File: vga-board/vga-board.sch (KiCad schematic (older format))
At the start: 44 parts, among them J1 Conn_02x20_Odd_Even, J2 Conn_02x20_Odd_Even, J3 DB15_Female_HighDensity, U1 74HC244, U10 74HC163, U11 74LS158, U12 74LS251, U13 74HC244, U14 74HC244, U15 74HC244, U16 GAL22V10, U17 GAL22V10, U18 GAL22V10, U19 74HC163, U2 74HC373, U20 74HC163, U21 74HC163, U22 74HC163, U23 74HC163, U3 74HC244, U4 74HC373, U5 74HC373, U6 74HC373, U7 74HC373, U8 71256SA12TPG, U9 74HC244, X1 40MHz

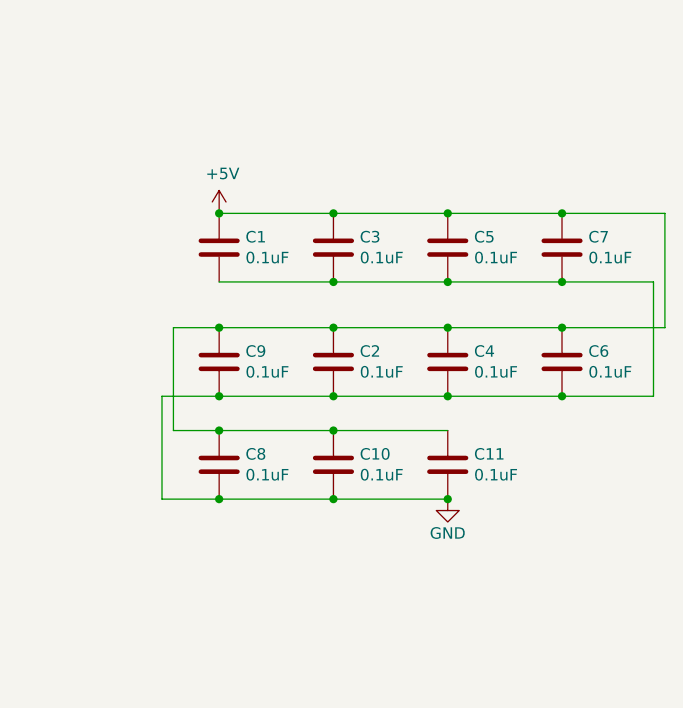
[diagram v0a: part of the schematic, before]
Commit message: Revert "More on layouts"
This reverts commit 3fc7c4d1a32f245eaa0a26aebed00be081417dbd.
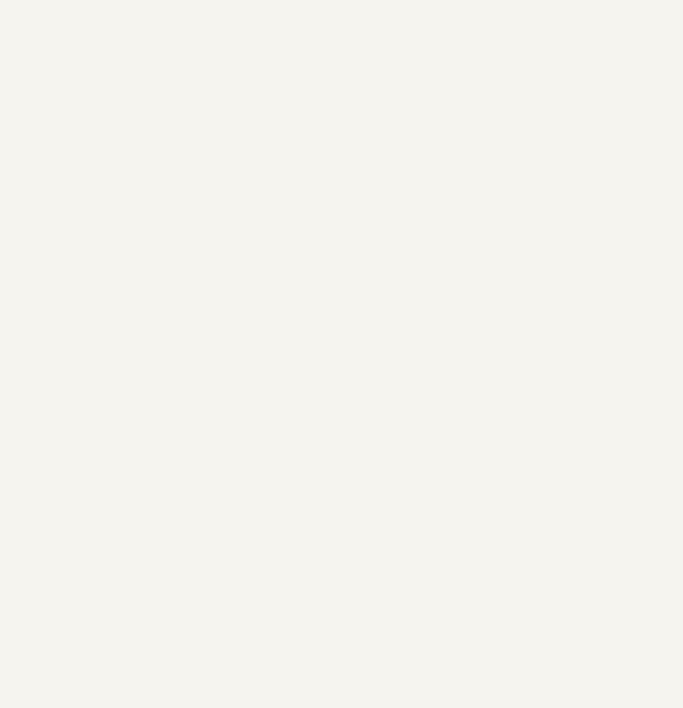
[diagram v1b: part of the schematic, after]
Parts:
- removed C1, C10, C11, C2, C3, C4, C5, C6, C7, C8, C9: 0.1uF, Capacitor_THT:C_Disc_D6.0mm_W2.5mm_P5.00mm, symbol Device:C
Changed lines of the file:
@@
 $EndComp
 NoConn ~ 14850 8500
-$Comp
-L Device:C C1
-U 1 1 5FE43840
-P 16900 2350
-F 0 "C1" H 17015 2396 50  0000 L CNN
-F 1 "0.1uF" H 17015 2305 50  0000 L CNN
-F 2 "Capacitor_THT:C_Disc_D6.0mm_W2.5mm_P5.00mm" H 16938 2200 50  0001 C CNN
-F 3 "~" H 16900 2350 50  0001 C CNN
-	1    16900 2350
-	1    0    0    -1
-$EndComp
-$Comp
-L Device:C C3
-U 1 1 5FE455E8
-P 17400 2350
-F 0 "C3" H 17515 2396 50  0000 L CNN
-F 1 "0.1uF" H 17515 2305 50  0000 L CNN
-F 2 "Capacitor_THT:C_Disc_D6.0mm_W2.5mm_P5.00mm" H 17438 2200 50  0001 C CNN
-F 3 "~" H 17400 2350 50  0001 C CNN
-	1    17400 2350
-	1    0    0    -1
-$EndComp
-$Comp
-L Device:C C5
-U 1 1 5FE4566B
-P 17900 2350
-F 0 "C5" H 18015 2396 50  0000 L CNN
-F 1 "0.1uF" H 18015 2305 50  0000 L CNN
-F 2 "Capacitor_THT:C_Disc_D6.0mm_W2.5mm_P5.00mm" H 17938 2200 50  0001 C CNN
-F 3 "~" H 17900 2350 50  0001 C CNN
-	1    17900 2350
-	1    0    0    -1
-$EndComp
-$Comp
-L Device:C C7
-U 1 1 5FE456D2
-P 18400 2350
-F 0 "C7" H 18515 2396 50  0000 L CNN
-F 1 "0.1uF" H 18515 2305 50  0000 L CNN
-F 2 "Capacitor_THT:C_Disc_D6.0mm_W2.5mm_P5.00mm" H 18438 2200 50  0001 C CNN
-F 3 "~" H 18400 2350 50  0001 C CNN
-	1    18400 2350
-	1    0    0    -1
-$EndComp
-$Comp
-L Device:C C9
-U 1 1 5FE45727
-P 16900 2850
-F 0 "C9" H 17015 2896 50  0000 L CNN
-F 1 "0.1uF" H 17015 2805 50  0000 L CNN
-F 2 "Capacitor_THT:C_Disc_D6.0mm_W2.5mm_P5.00mm" H 16938 2700 50  0001 C CNN
-F 3 "~" H 16900 2850 50  0001 C CNN
-	1    16900 2850
-	1    0    0    -1
-$EndComp
-$Comp
-L Device:C C2
-U 1 1 5FE4577C
-P 17400 2850
-F 0 "C2" H 17515 2896 50  0000 L CNN
-F 1 "0.1uF" H 17515 2805 50  0000 L CNN
-F 2 "Capacitor_THT:C_Disc_D6.0mm_W2.5mm_P5.00mm" H 17438 2700 50  0001 C CNN
-F 3 "~" H 17400 2850 50  0001 C CNN
-	1    17400 2850
-	1    0    0    -1
-$EndComp
-$Comp
-L Device:C C4
-U 1 1 5FE457D6
-P 17900 2850
-F 0 "C4" H 18015 2896 50  0000 L CNN
-F 1 "0.1uF" H 18015 2805 50  0000 L CNN
-F 2 "Capacitor_THT:C_Disc_D6.0mm_W2.5mm_P5.00mm" H 17938 2700 50  0001 C CNN
-F 3 "~" H 17900 2850 50  0001 C CNN
-	1    17900 2850
-	1    0    0    -1
-$EndComp
-$Comp
-L Device:C C6
-U 1 1 5FE45854
-P 18400 2850
-F 0 "C6" H 18515 2896 50  0000 L CNN
-F 1 "0.1uF" H 18515 2805 50  0000 L CNN
-F 2 "Capacitor_THT:C_Disc_D6.0mm_W2.5mm_P5.00mm" H 18438 2700 50  0001 C CNN
-F 3 "~" H 18400 2850 50  0001 C CNN
-	1    18400 2850
-	1    0    0    -1
-$EndComp
-$Comp
-L Device:C C8
-U 1 1 5FE458A9
-P 16900 3300
-F 0 "C8" H 17015 3346 50  0000 L CNN
-F 1 "0.1uF" H 17015 3255 50  0000 L CNN
-F 2 "Capacitor_THT:C_Disc_D6.0mm_W2.5mm_P5.00mm" H 16938 3150 50  0001 C CNN
-F 3 "~" H 16900 3300 50  0001 C CNN
-	1    16900 3300
-	1    0    0    -1
-$EndComp
-$Comp
-L Device:C C10
-U 1 1 5FE458FE
-P 17400 3300
-F 0 "C10" H 17515 3346 50  0000 L CNN
-F 1 "0.1uF" H 17515 3255 50  0000 L CNN
-F 2 "Capacitor_THT:C_Disc_D6.0mm_W2.5mm_P5.00mm" H 17438 3150 50  0001 C CNN
-F 3 "~" H 17400 3300 50  0001 C CNN
-	1    17400 3300
-	1    0    0    -1
-$EndComp
-$Comp
-L Device:C C11
-U 1 1 5FE9F61C
-P 17900 3300
-F 0 "C11" H 18015 3346 50  0000 L CNN
-F 1 "0.1uF" H 18015 3255 50  0000 L CNN
-F 2 "Capacitor_THT:C_Disc_D6.0mm_W2.5mm_P5.00mm" H 17938 3150 50  0001 C CNN
-F 3 "~" H 17900 3300 50  0001 C CNN
-	1    17900 3300
-	1    0    0    -1
-$EndComp
-Wire Wire Line
-	16900 2200 17400 2200
-Connection ~ 17400 2200
-Wire Wire Line
-	17400 2200 17900 2200
-Connection ~ 17900 2200
-Wire Wire Line
-	17900 2200 18400 2200
-Wire Wire Line
-	18400 2200 18850 2200
-Wire Wire Line
-	18850 2200 18850 2700
-Wire Wire Line
-	18850 2700 18400 2700
-Connection ~ 18400 2200
-Connection ~ 17900 2700
-Wire Wire Line
-	17900 2700 17400 2700
-Connection ~ 18400 2700
-Wire Wire Line
-	18400 2700 17900 2700
-Wire Wire Line
-	17400 2700 16900 2700
-Wire Wire Line
-	16700 2700 16700 3150
-Wire Wire Line
-	16700 3150 16900 3150
-Connection ~ 17400 2700
-Connection ~ 16900 2700
-Wire Wire Line
-	16900 2700 16700 2700
-Connection ~ 16900 3150
-Wire Wire Line
-	16900 3150 17400 3150
-Connection ~ 17400 3150
-Wire Wire Line
-	17400 3150 17900 3150
-Wire Wire Line
-	16900 2500 17400 2500
-Wire Wire Line
-	18800 2500 18800 3000
-Wire Wire Line
-	18800 3000 18400 3000
-Wire Wire Line
-	16650 3000 16650 3450
-Wire Wire Line
-	16650 3450 16900 3450
-Connection ~ 17400 2500
-Wire Wire Line
-	17400 2500 17900 2500
-Connection ~ 17900 2500
-Wire Wire Line
-	17900 2500 18400 2500
-Connection ~ 18400 2500
-Wire Wire Line
-	18400 2500 18800 2500
-Connection ~ 16900 3000
-Wire Wire Line
-	16900 3000 16650 3000
-Connection ~ 17400 3000
-Wire Wire Line
-	17400 3000 16900 3000
-Connection ~ 17900 3000
-Wire Wire Line
-	17900 3000 17400 3000
-Connection ~ 18400 3000
-Wire Wire Line
-	18400 3000 17900 3000
-Connection ~ 16900 3450
-Wire Wire Line
-	16900 3450 17400 3450
-Connection ~ 17400 3450
-Wire Wire Line
-	17400 3450 17900 3450
-Connection ~ 17900 3450
-$Comp
-L power:+5V #PWR0173
-U 1 1 5FEBEE51
-P 16900 2200
-F 0 "#PWR0173" H 16900 2050 50  0001 C CNN
-F 1 "+5V" H 16915 2373 50  0000 C CNN
-F 2 "" H 16900 2200 50  0001 C CNN
-F 3 "" H 16900 2200 50  0001 C CNN
-	1    16900 2200
-	1    0    0    -1
-$EndComp
-Connection ~ 16900 2200
-$Comp
-L power:GND #PWR0174
-U 1 1 5FEBF844
-P 17900 3450
-F 0 "#PWR0174" H 17900 3200 50  0001 C CNN
-F 1 "GND" H 17900 3300 50  0000 C CNN
-F 2 "" H 17900 3450 50  0001 C CNN
-F 3 "" H 17900 3450 50  0001 C CNN
-	1    17900 3450
-	1    0    0    -1
-$EndComp
 $EndSCHEMATC

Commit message: More on layouts
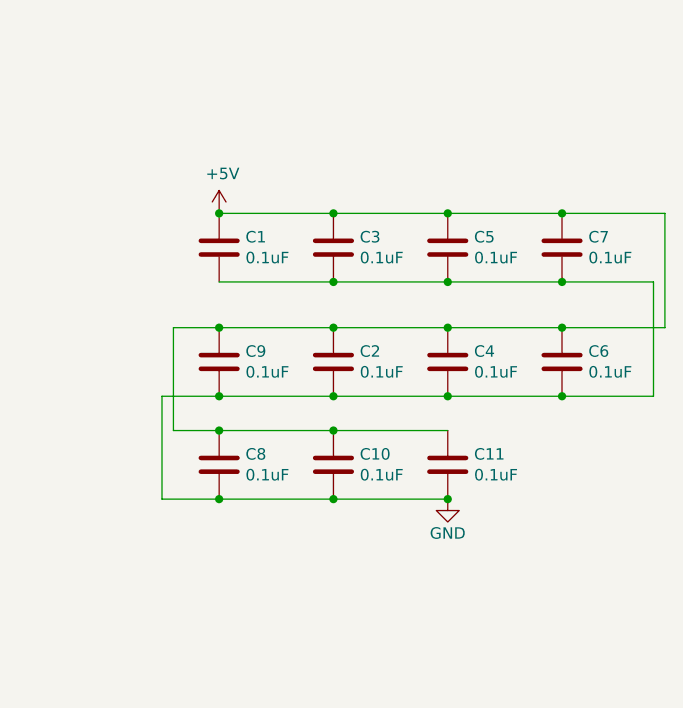
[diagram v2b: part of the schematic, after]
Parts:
- added C1, C10, C11, C2, C3, C4, C5, C6, C7, C8, C9: 0.1uF, Capacitor_THT:C_Disc_D6.0mm_W2.5mm_P5.00mm, symbol Device:C
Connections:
- net +5V: now also C1.1, C10.1, C11.1, C2.1, C3.1, C4.1, C5.1, C6.1, C7.1, C8.1, C9.1
- net GND: now also C1.2, C10.2, C11.2, C2.2, C3.2, C4.2, C5.2, C6.2, C7.2, C8.2, C9.2
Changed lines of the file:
@@
 $EndComp
 NoConn ~ 14850 8500
+$Comp
+L Device:C C1
+U 1 1 5FE43840
+P 16900 2350
+F 0 "C1" H 17015 2396 50  0000 L CNN
+F 1 "0.1uF" H 17015 2305 50  0000 L CNN
+F 2 "Capacitor_THT:C_Disc_D6.0mm_W2.5mm_P5.00mm" H 16938 2200 50  0001 C CNN
+F 3 "~" H 16900 2350 50  0001 C CNN
+	1    16900 2350
+	1    0    0    -1
+$EndComp
+$Comp
+L Device:C C3
+U 1 1 5FE455E8
+P 17400 2350
+F 0 "C3" H 17515 2396 50  0000 L CNN
+F 1 "0.1uF" H 17515 2305 50  0000 L CNN
+F 2 "Capacitor_THT:C_Disc_D6.0mm_W2.5mm_P5.00mm" H 17438 2200 50  0001 C CNN
+F 3 "~" H 17400 2350 50  0001 C CNN
+	1    17400 2350
+	1    0    0    -1
+$EndComp
+$Comp
+L Device:C C5
+U 1 1 5FE4566B
+P 17900 2350
+F 0 "C5" H 18015 2396 50  0000 L CNN
+F 1 "0.1uF" H 18015 2305 50  0000 L CNN
+F 2 "Capacitor_THT:C_Disc_D6.0mm_W2.5mm_P5.00mm" H 17938 2200 50  0001 C CNN
+F 3 "~" H 17900 2350 50  0001 C CNN
+	1    17900 2350
+	1    0    0    -1
+$EndComp
+$Comp
+L Device:C C7
+U 1 1 5FE456D2
+P 18400 2350
+F 0 "C7" H 18515 2396 50  0000 L CNN
+F 1 "0.1uF" H 18515 2305 50  0000 L CNN
+F 2 "Capacitor_THT:C_Disc_D6.0mm_W2.5mm_P5.00mm" H 18438 2200 50  0001 C CNN
+F 3 "~" H 18400 2350 50  0001 C CNN
+	1    18400 2350
+	1    0    0    -1
+$EndComp
+$Comp
+L Device:C C9
+U 1 1 5FE45727
+P 16900 2850
+F 0 "C9" H 17015 2896 50  0000 L CNN
+F 1 "0.1uF" H 17015 2805 50  0000 L CNN
+F 2 "Capacitor_THT:C_Disc_D6.0mm_W2.5mm_P5.00mm" H 16938 2700 50  0001 C CNN
+F 3 "~" H 16900 2850 50  0001 C CNN
+	1    16900 2850
+	1    0    0    -1
+$EndComp
+$Comp
+L Device:C C2
+U 1 1 5FE4577C
+P 17400 2850
+F 0 "C2" H 17515 2896 50  0000 L CNN
+F 1 "0.1uF" H 17515 2805 50  0000 L CNN
+F 2 "Capacitor_THT:C_Disc_D6.0mm_W2.5mm_P5.00mm" H 17438 2700 50  0001 C CNN
+F 3 "~" H 17400 2850 50  0001 C CNN
+	1    17400 2850
+	1    0    0    -1
+$EndComp
+$Comp
+L Device:C C4
+U 1 1 5FE457D6
+P 17900 2850
+F 0 "C4" H 18015 2896 50  0000 L CNN
+F 1 "0.1uF" H 18015 2805 50  0000 L CNN
+F 2 "Capacitor_THT:C_Disc_D6.0mm_W2.5mm_P5.00mm" H 17938 2700 50  0001 C CNN
+F 3 "~" H 17900 2850 50  0001 C CNN
+	1    17900 2850
+	1    0    0    -1
+$EndComp
+$Comp
+L Device:C C6
+U 1 1 5FE45854
+P 18400 2850
+F 0 "C6" H 18515 2896 50  0000 L CNN
+F 1 "0.1uF" H 18515 2805 50  0000 L CNN
+F 2 "Capacitor_THT:C_Disc_D6.0mm_W2.5mm_P5.00mm" H 18438 2700 50  0001 C CNN
+F 3 "~" H 18400 2850 50  0001 C CNN
+	1    18400 2850
+	1    0    0    -1
+$EndComp
+$Comp
+L Device:C C8
+U 1 1 5FE458A9
+P 16900 3300
+F 0 "C8" H 17015 3346 50  0000 L CNN
+F 1 "0.1uF" H 17015 3255 50  0000 L CNN
+F 2 "Capacitor_THT:C_Disc_D6.0mm_W2.5mm_P5.00mm" H 16938 3150 50  0001 C CNN
+F 3 "~" H 16900 3300 50  0001 C CNN
+	1    16900 3300
+	1    0    0    -1
+$EndComp
+$Comp
+L Device:C C10
+U 1 1 5FE458FE
+P 17400 3300
+F 0 "C10" H 17515 3346 50  0000 L CNN
+F 1 "0.1uF" H 17515 3255 50  0000 L CNN
+F 2 "Capacitor_THT:C_Disc_D6.0mm_W2.5mm_P5.00mm" H 17438 3150 50  0001 C CNN
+F 3 "~" H 17400 3300 50  0001 C CNN
+	1    17400 3300
+	1    0    0    -1
+$EndComp
+$Comp
+L Device:C C11
+U 1 1 5FE9F61C
+P 17900 3300
+F 0 "C11" H 18015 3346 50  0000 L CNN
+F 1 "0.1uF" H 18015 3255 50  0000 L CNN
+F 2 "Capacitor_THT:C_Disc_D6.0mm_W2.5mm_P5.00mm" H 17938 3150 50  0001 C CNN
+F 3 "~" H 17900 3300 50  0001 C CNN
+	1    17900 3300
+	1    0    0    -1
+$EndComp
+Wire Wire Line
+	16900 2200 17400 2200
+Connection ~ 17400 2200
+Wire Wire Line
+	17400 2200 17900 2200
+Connection ~ 17900 2200
+Wire Wire Line
+	17900 2200 18400 2200
+Wire Wire Line
+	18400 2200 18850 2200
+Wire Wire Line
+	18850 2200 18850 2700
+Wire Wire Line
+	18850 2700 18400 2700
+Connection ~ 18400 2200
+Connection ~ 17900 2700
+Wire Wire Line
+	17900 2700 17400 2700
+Connection ~ 18400 2700
+Wire Wire Line
+	18400 2700 17900 2700
+Wire Wire Line
+	17400 2700 16900 2700
+Wire Wire Line
+	16700 2700 16700 3150
+Wire Wire Line
+	16700 3150 16900 3150
+Connection ~ 17400 2700
+Connection ~ 16900 2700
+Wire Wire Line
+	16900 2700 16700 2700
+Connection ~ 16900 3150
+Wire Wire Line
+	16900 3150 17400 3150
+Connection ~ 17400 3150
+Wire Wire Line
+	17400 3150 17900 3150
+Wire Wire Line
+	16900 2500 17400 2500
+Wire Wire Line
+	18800 2500 18800 3000
+Wire Wire Line
+	18800 3000 18400 3000
+Wire Wire Line
+	16650 3000 16650 3450
+Wire Wire Line
+	16650 3450 16900 3450
+Connection ~ 17400 2500
+Wire Wire Line
+	17400 2500 17900 2500
+Connection ~ 17900 2500
+Wire Wire Line
+	17900 2500 18400 2500
+Connection ~ 18400 2500
+Wire Wire Line
+	18400 2500 18800 2500
+Connection ~ 16900 3000
+Wire Wire Line
+	16900 3000 16650 3000
+Connection ~ 17400 3000
+Wire Wire Line
+	17400 3000 16900 3000
+Connection ~ 17900 3000
+Wire Wire Line
+	17900 3000 17400 3000
+Connection ~ 18400 3000
+Wire Wire Line
+	18400 3000 17900 3000
+Connection ~ 16900 3450
+Wire Wire Line
+	16900 3450 17400 3450
+Connection ~ 17400 3450
+Wire Wire Line
+	17400 3450 17900 3450
+Connection ~ 17900 3450
+$Comp
+L power:+5V #PWR0173
+U 1 1 5FEBEE51
+P 16900 2200
+F 0 "#PWR0173" H 16900 2050 50  0001 C CNN
+F 1 "+5V" H 16915 2373 50  0000 C CNN
+F 2 "" H 16900 2200 50  0001 C CNN
+F 3 "" H 16900 2200 50  0001 C CNN
+	1    16900 2200
+	1    0    0    -1
+$EndComp
+Connection ~ 16900 2200
+$Comp
+L power:GND #PWR0174
+U 1 1 5FEBF844
+P 17900 3450
+F 0 "#PWR0174" H 17900 3200 50  0001 C CNN
+F 1 "GND" H 17900 3300 50  0000 C CNN
+F 2 "" H 17900 3450 50  0001 C CNN
+F 3 "" H 17900 3450 50  0001 C CNN
+	1    17900 3450
+	1    0    0    -1
+$EndComp
 $EndSCHEMATC
